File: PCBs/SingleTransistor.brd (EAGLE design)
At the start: 20.5 x 32.5 mm, 4 parts, among them T1 BC547N

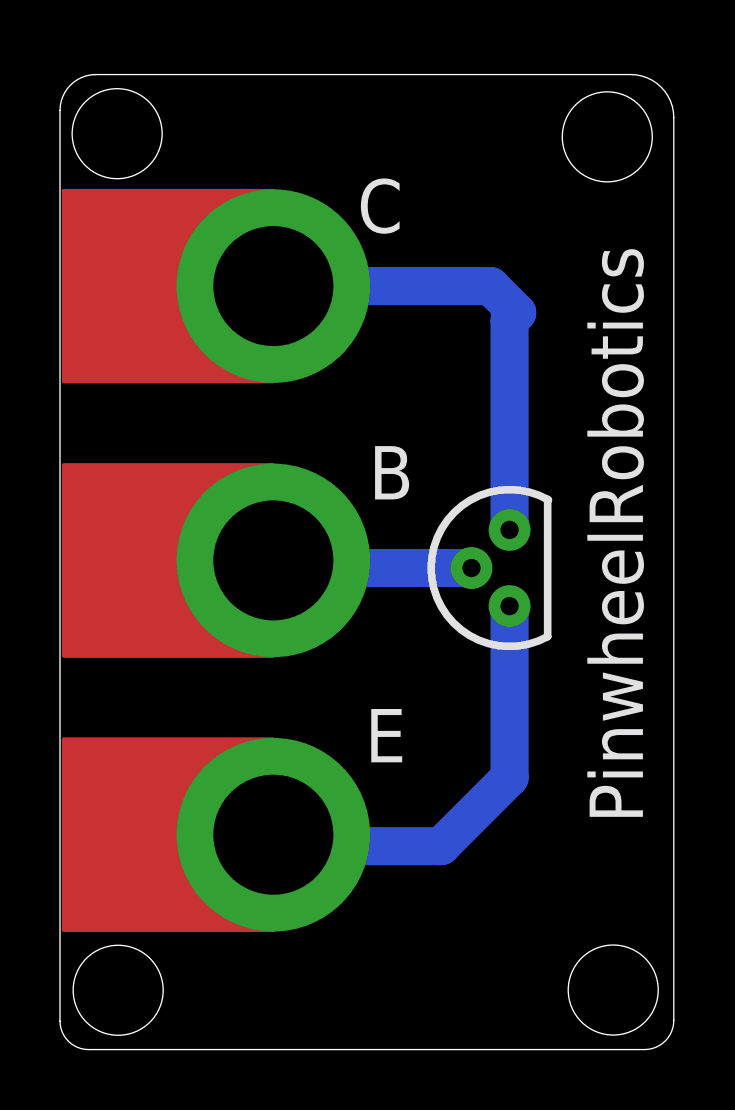
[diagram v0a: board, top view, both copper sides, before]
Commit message: New Update
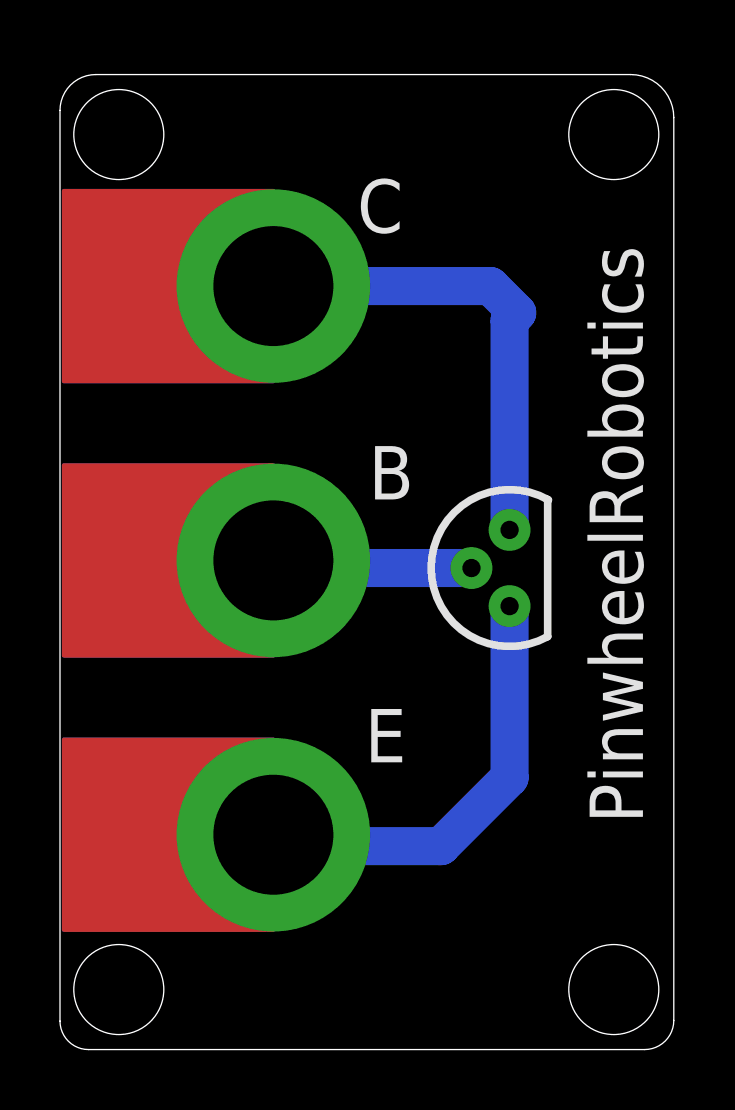
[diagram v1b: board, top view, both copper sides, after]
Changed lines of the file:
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@@
 <drawing>
 <settings>
-<setting alwaysvectorfont="yes"/>
+<setting alwaysvectorfont="no"/>
 <setting verticaltext="up"/>
 </settings>
@@
 <text x="12.827" y="29.337" size="1.778" layer="21">B</text>
 <text x="12.446" y="38.227" size="1.778" layer="21">C</text>
-<hole x="4.445" y="41.529" drill="3"/>
-<hole x="20.783" y="41.423" drill="3"/>
-<hole x="20.981" y="12.984" drill="3"/>
-<hole x="4.479" y="12.976" drill="3"/>
+<hole x="4.5" y="41.5" drill="3"/>
+<hole x="21" y="41.5" drill="3"/>
+<hole x="21" y="13" drill="3"/>
+<hole x="4.5" y="13" drill="3"/>
 <text x="21.971" y="18.542" size="1.778" layer="21" rot="R90">PinwheelRobotics</text>
 <text x="21.971" y="37.465" size="1.778" layer="22" rot="MR270">care@pinwheel.in</text>
